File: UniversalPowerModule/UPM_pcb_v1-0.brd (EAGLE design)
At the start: 39.4 x 25.4 mm, 27 parts, among them Q1 DMP4047SK3, U1 TLV1117_4TERM-33_DCY, U2 TLV1117_4TERM-50_DCY

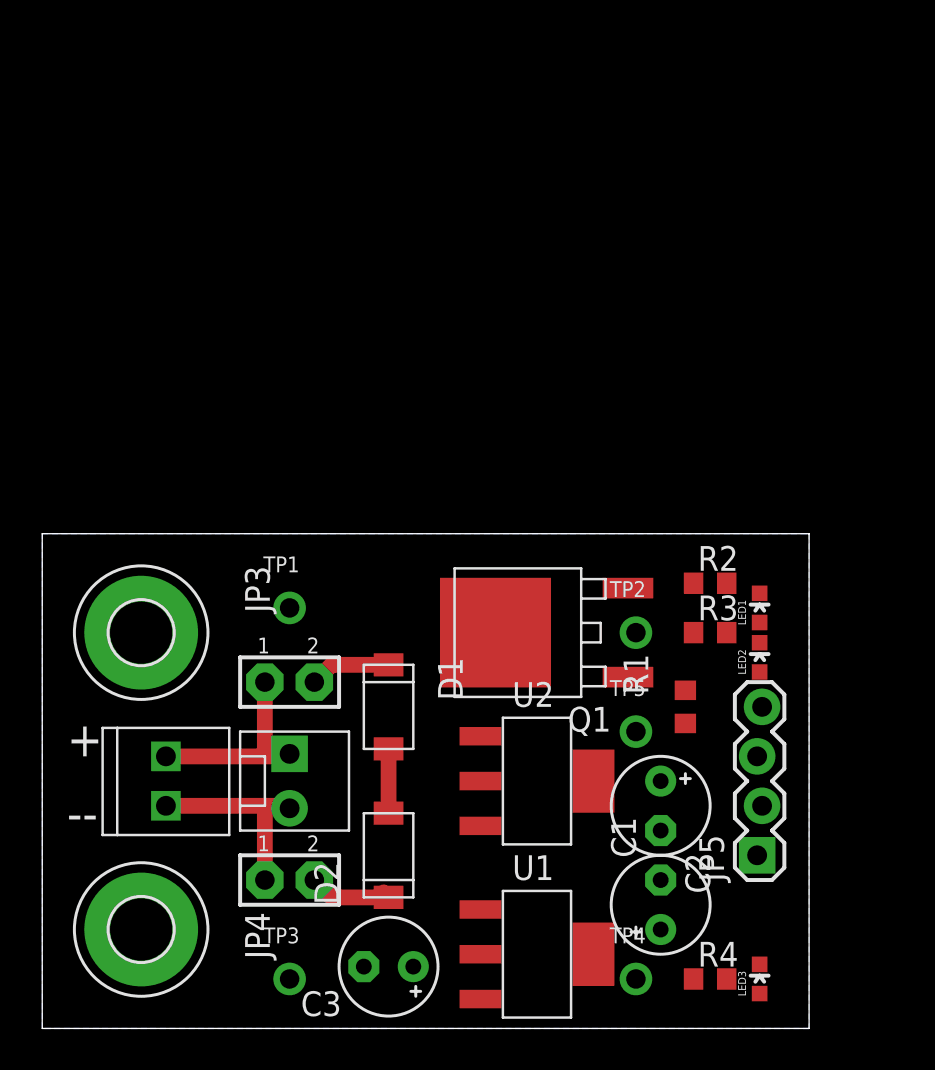
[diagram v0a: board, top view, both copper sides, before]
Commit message: UPM+CAN v1 sent to FAB
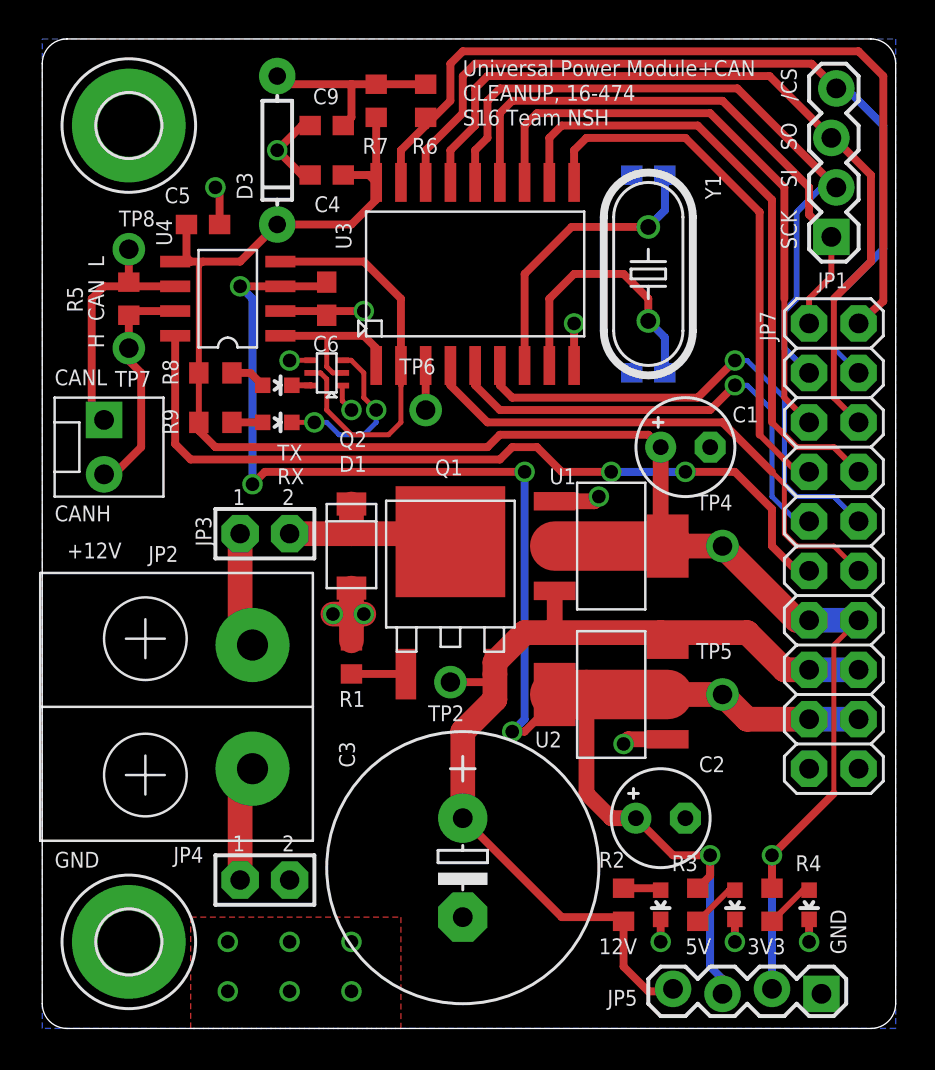
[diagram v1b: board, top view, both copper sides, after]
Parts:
- removed D2: VISHAY_SMA6F, npol-discrete:VSHY_DO-221AC
- removed TP1, TP3: (no value), microbuilder:1X01_ROUND
- added C4, C5, C6: 0.1uF, rcl:C0603
- added C7, C8: 22nF, rcl:C0603
- added C9: 10nF, rcl:C0603
- added D3: (no value), SparkFun-DiscreteSemi:DIODE-1N4148
- added JP6: M02POLAR_LOCK, SparkFun-Connectors:MOLEX-1X2_LOCK
- added JP7: M10X2, SparkFun-Connectors:2X10
- added LED4: green, SparkFun-LED:LED-0603
- added LED5: blue, SparkFun-LED:LED-0603
- added Q2: INFINEON_2N7002_DW, npol-discrete:INFINEON_SOT363
- added R5: 120, rcl:R0603
- added R6, R7: 10k, rcl:R0603
- added R8, R9: 330, rcl:R0603
- added TP6, TP7, TP8: (no value), microbuilder:1X01_ROUND
- added U3: MCP2515-SO, npol-digital:MCP_SO_SOIC-18
- added U4: MCP2562-SN, npol-digital:MCP_SN_SOIC-8
- added Y1: 8MHz, SparkFun-FreqCtrl:HC49U-V
- C3: value 100uF -> 1000uF; device rcl:E2,5-5 -> rcl:E5-13
- JP1: value M022.54MM_SCREWTERM -> (none); device SparkFun-Connectors:1X02_2.54_SCREWTERM -> SparkFun-Connectors:1X04_LOCK
- JP2: value M02POLAR_LOCK -> ONSHORE_OSTYK21102030; device SparkFun-Connectors:MOLEX-1X2_LOCK -> npol-connectors:ONSHORE_OSTYK21102030
- moved JP1 45.0 mm to (40.6, 40.6)
- moved H2 26.0 mm to (4.45, 46.4)
- moved C1 23.5 mm to (33.0, 29.8), turned to 0 degrees
- moved TP4 22.7 mm to (34.9, 24.8)
- moved U1 21.3 mm to (29.2, 24.8)
- moved R1 17.3 mm to (15.9, 19.1), turned to 270 degrees
- moved R2 17.1 mm to (29.8, 6.35), turned to 270 degrees
- moved LED1 16.1 mm to (31.8, 6.35), turned to 180 degrees
- moved R3 14.0 mm to (33.7, 6.35), turned to 90 degrees
- moved LED2 12.8 mm to (35.6, 6.35), turned to 180 degrees
- moved TP2 9.86 mm to (21.0, 17.8)
- moved D1 8.47 mm to (15.9, 24.8)
- moved JP3 7.73 mm to (12.7, 25.4)
- moved JP5 7.67 mm to (40.0, 1.91), turned to 180 degrees
- moved C3 6.35 mm to (21.6, 8.26), turned to 270 degrees
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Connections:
- removed net +3.3V: C1.+, JP5.2, R4.2, TP4.1, U1.2, U1.4
- new net +3V3: C1.+, C4.1, C5.1, D3.C, JP5.2, JP7.13, JP7.14, R4.2, R7.2, R8.1, R9.1, TP4.1, U1.2, U1.4, U3.18, U4.5
- new net /CS: JP1.4, JP7.4, U3.16
- new net /INT: JP7.5, U3.12
- new net /RESET: JP7.2, R6.2, U3.17
- new net /RX0BF: JP7.8, U3.11
- new net /RX1BF: JP7.7, U3.10
- new net /TX0RTS: JP7.12, U3.4
- new net /TX1RTS: JP7.9, U3.5
- new net /TX2RTS: JP7.10, U3.6
- new net CANH: JP6.2, R5.2, TP7.1, U4.7
- new net CANL: JP6.1, R5.1, TP8.1, U4.6
- new net CLKOUT: TP6.1, U3.3
- new net MISO: JP1.3, JP7.6, U3.15
- new net MOSI: JP1.2, JP7.3, U3.14
- new net N$10: LED4.A, R8.2
- new net N$11: LED5.A, R9.2
- new net N$7: C9.1, D3.A, R6.1, R7.1
- new net N$8: LED5.C, Q2.3
- new net RXCAN: Q2.5, U3.2, U4.4
- new net SCK: JP1.1, JP7.1, U3.13
- new net STBY: JP7.11, U4.8
- new net TXCAN: Q2.2, U3.1, U4.1
- new net XTAL1: C8.1, U3.8, Y1.2
- new net XTAL2: C7.1, U3.7, Y1.1
- net +12V: now also JP7.15, JP7.16
- net +5V: now also C6.1, JP7.17, JP7.18, U4.3
- net GND: now also C4.2, C5.2, C6.2, C7.2, C8.2, C9.2, D1.A, JP7.19, JP7.20, Q2.1, Q2.4, U3.9, U4.2; no longer D2.K, TP3.1
- net N$1: now also LED4.C, Q2.6; no longer D1.A, D2.A
- net VIN+: now also JP2.2; no longer JP1.P1, JP2.1, TP1.1
- net VIN-: now also JP2.1; no longer JP1.P2, JP2.2
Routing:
- net +3V3: track 0.00 -> 97.9 mm, vias 0 -> 1
- net +5V: track 0.00 -> 84.2 mm, vias 0 -> 5
- net +12V: track 0.00 -> 50.4 mm
- net /RESET: track 0.00 -> 43.8 mm
- net /CS: track 0.00 -> 43.7 mm
- net STBY: track 0.00 -> 42.4 mm, vias 0 -> 2
- net MISO: track 0.00 -> 42.1 mm
- net MOSI: track 0.00 -> 36.3 mm
- net /RX0BF: track 0.00 -> 32.5 mm
- net /INT: track 0.00 -> 30.7 mm
- net SCK: track 0.00 -> 29.5 mm
- net /RX1BF: track 0.00 -> 27.8 mm
- net /TX0RTS: track 0.00 -> 27.4 mm
- net /TX2RTS: track 0.00 -> 26.5 mm, vias 0 -> 1
- net /TX1RTS: track 0.00 -> 24.7 mm, vias 0 -> 1
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- added copper zone on layer 1, net GND
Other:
- board size 39.4 x 25.4 mm -> 43.8 x 50.8 mm
- board text added: "+12V"
- board text added: "/CS"
- board text added: "12V"
- board text added: "3V3"
- board text added: "5V"
- board text added: "CANH"
- board text added: "CANL"
- board text added: "CLEANUP, 16-474"
- board text added: "GND"
- board text added: "H CAN L"
- board text added: "S16 Team NSH"
- board text added: "SCK"
- board text added: "SI"
- board text added: "SO"
- board text added: "TX RX"
- board text added: "Universal Power Module+CAN"
- board text removed: "+"
- board text removed: "--"
